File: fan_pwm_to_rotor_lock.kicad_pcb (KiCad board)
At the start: 2 copper layers, 69 x 40.5 mm, 12 parts, among them J1 Conn_01x04, J2 Conn_01x04, U1 LM393

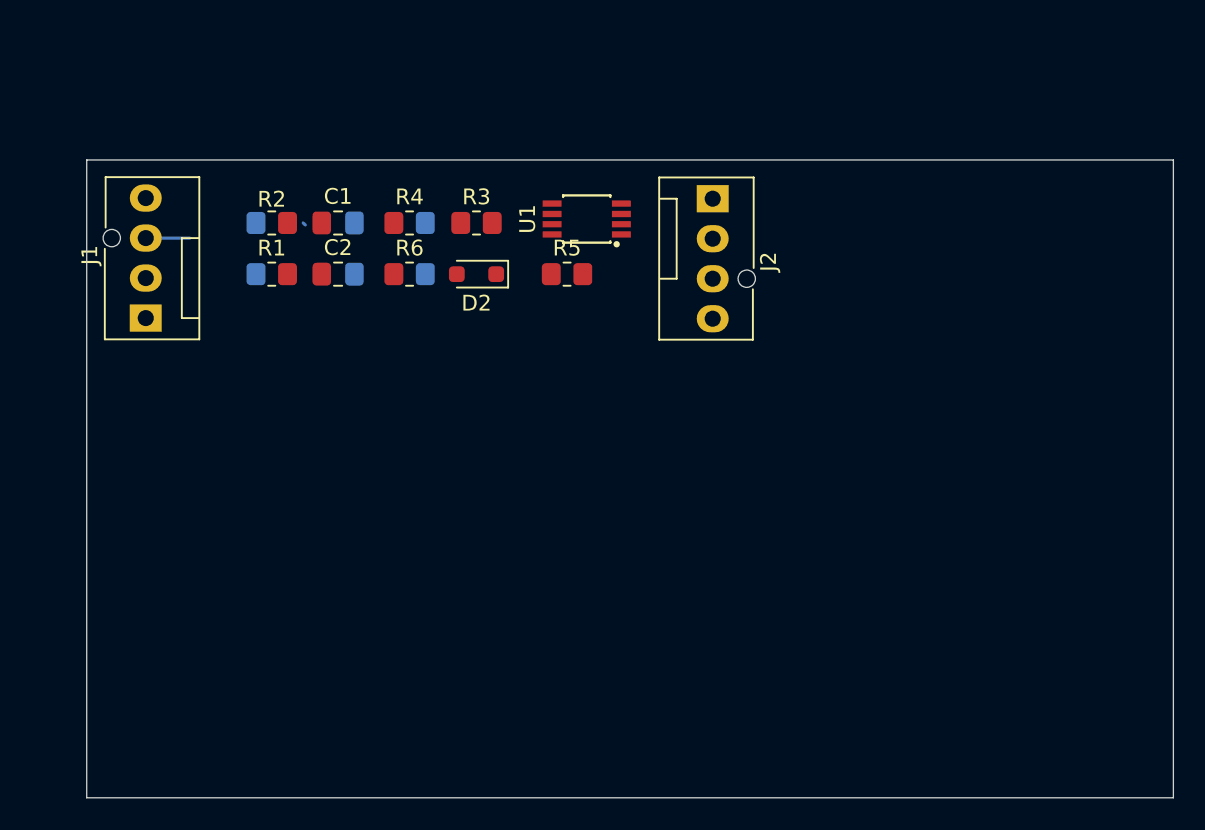
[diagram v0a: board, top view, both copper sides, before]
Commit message: update
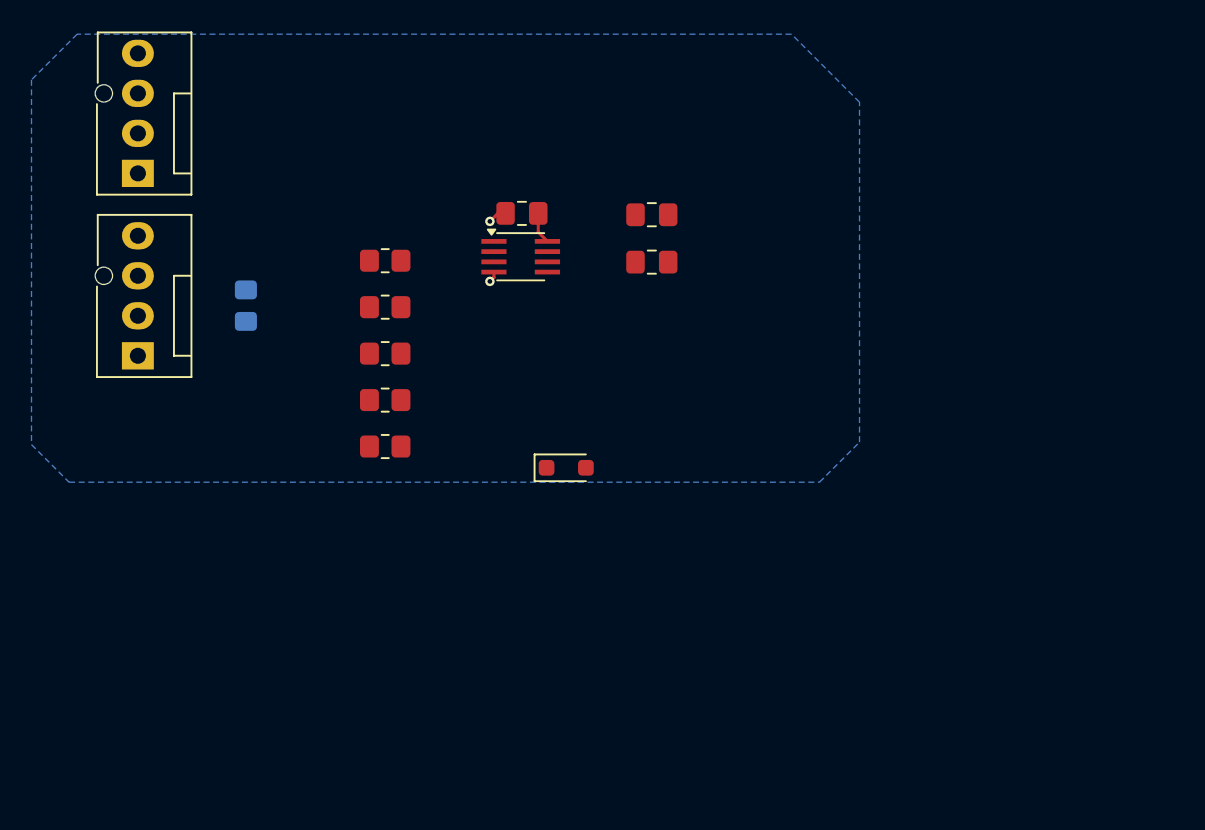
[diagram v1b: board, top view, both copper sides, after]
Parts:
- added C3: 100n, Capacitor_SMD:C_0805_2012Metric_Pad1.18x1.45mm_HandSolder, F.Cu at (56.1, 24.9)
- R1: moved to B.Cu
- U1: footprint easyeda2kicad:MINISO-8_L3.0-W3.0-P0.65-LS4.9-BL -> Package_SO:SSOP-8_2.95x2.8mm_P0.65mm
- moved J2 36.5 mm to (31.8, 22.4), turned to 90 degrees
- moved C2 19.9 mm to (64.4, 28.0)
- moved C1 19.9 mm to (64.4, 25.0)
- moved R5 14.0 mm to (47.5, 36.7)
- moved D2 13.6 mm to (58.9, 41.0), turned to 0 degrees
- moved R6 11.1 mm to (47.5, 39.7)
- moved R4 8.44 mm to (47.5, 33.8)
- moved R3 7.89 mm to (47.5, 30.8)
- moved R2 7.59 mm to (47.5, 27.9)
- moved U1 4.83 mm to (56.1, 27.6), turned to 0 degrees
- moved R1 2.59 mm to (38.6, 30.8), turned to 90 degrees
- moved J1 2.45 mm to (31.8, 33.9)
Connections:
- J1 pad 4: unconnected-(J1-Pin_4-Pad4) -> /passthrough
- J2 pad 4: unconnected-(J2-Pin_4-Pad4) -> /passthrough
- R1 pad 1: VDD -> Net-(J1-Pin_1)
- R1 pad 2: Net-(J1-Pin_1) -> VDD
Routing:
- net VDD: track 0.00 -> 2.02 mm
- net GND: track 2.97 -> 1.90 mm, vias 0 -> 2
- added copper zone on B.Cu, net GND
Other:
- board outline removed
